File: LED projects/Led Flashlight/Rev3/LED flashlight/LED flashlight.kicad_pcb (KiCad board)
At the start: 2 copper layers, 39.5 x 19.4 mm, 10 parts

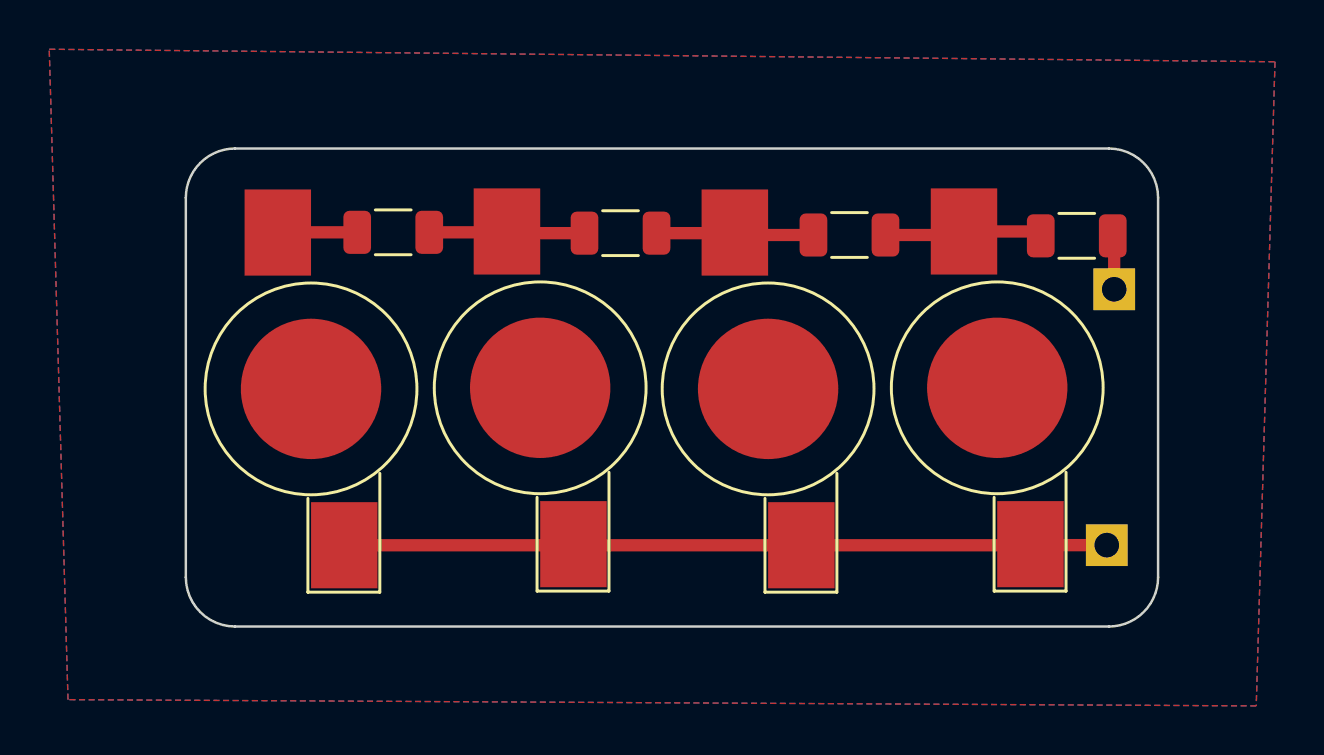
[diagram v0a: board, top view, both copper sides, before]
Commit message: update
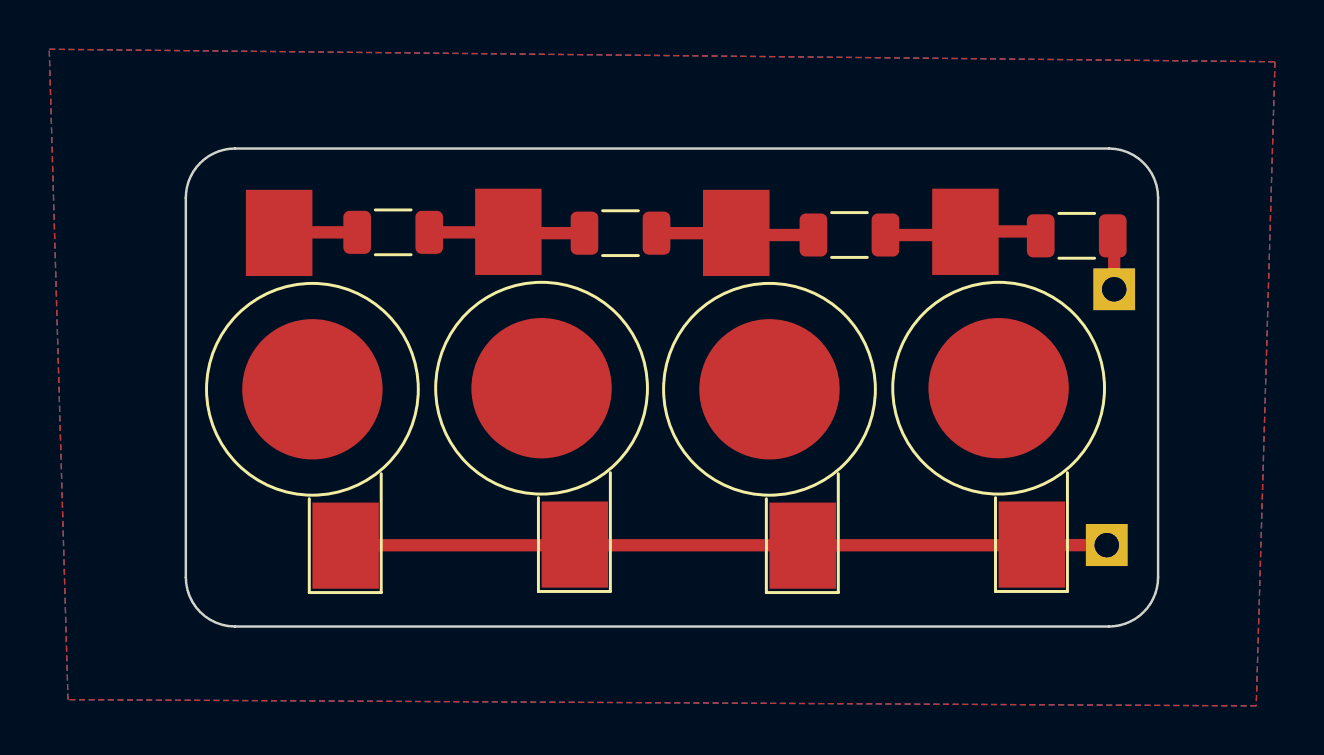
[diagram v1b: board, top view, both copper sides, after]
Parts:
- REF** (x4): value LED_1W_3W_R8 -> led1wsmdpersonal; footprint LED_SMD:LED_1W_3W_R8 -> personal:led1wsmdpersonal
